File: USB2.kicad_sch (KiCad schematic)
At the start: 0 parts

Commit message: usb work cont
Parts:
- added P1: USB_C_Plug_USB2.0, symbol Connector:USB_C_Plug_USB2.0
- added U2: TUSB2046BIVFR, TUSB2046BIVFR:QFP80P900X900X145-32N, symbol TUSB2046BIVFR:TUSB2046BIVFR
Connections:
- new net: P1.A1 (GND), P1.A12 (GND), P1.B1 (GND), P1.B12 (GND)
- new net: P1.A4 (VBUS), P1.A9 (VBUS), P1.B4 (VBUS), P1.B9 (VBUS)
- new net USB2_HOST2_DM: U2.2 (DM0)
- new net USB2_HOST2_DP: U2.1 (DP0)

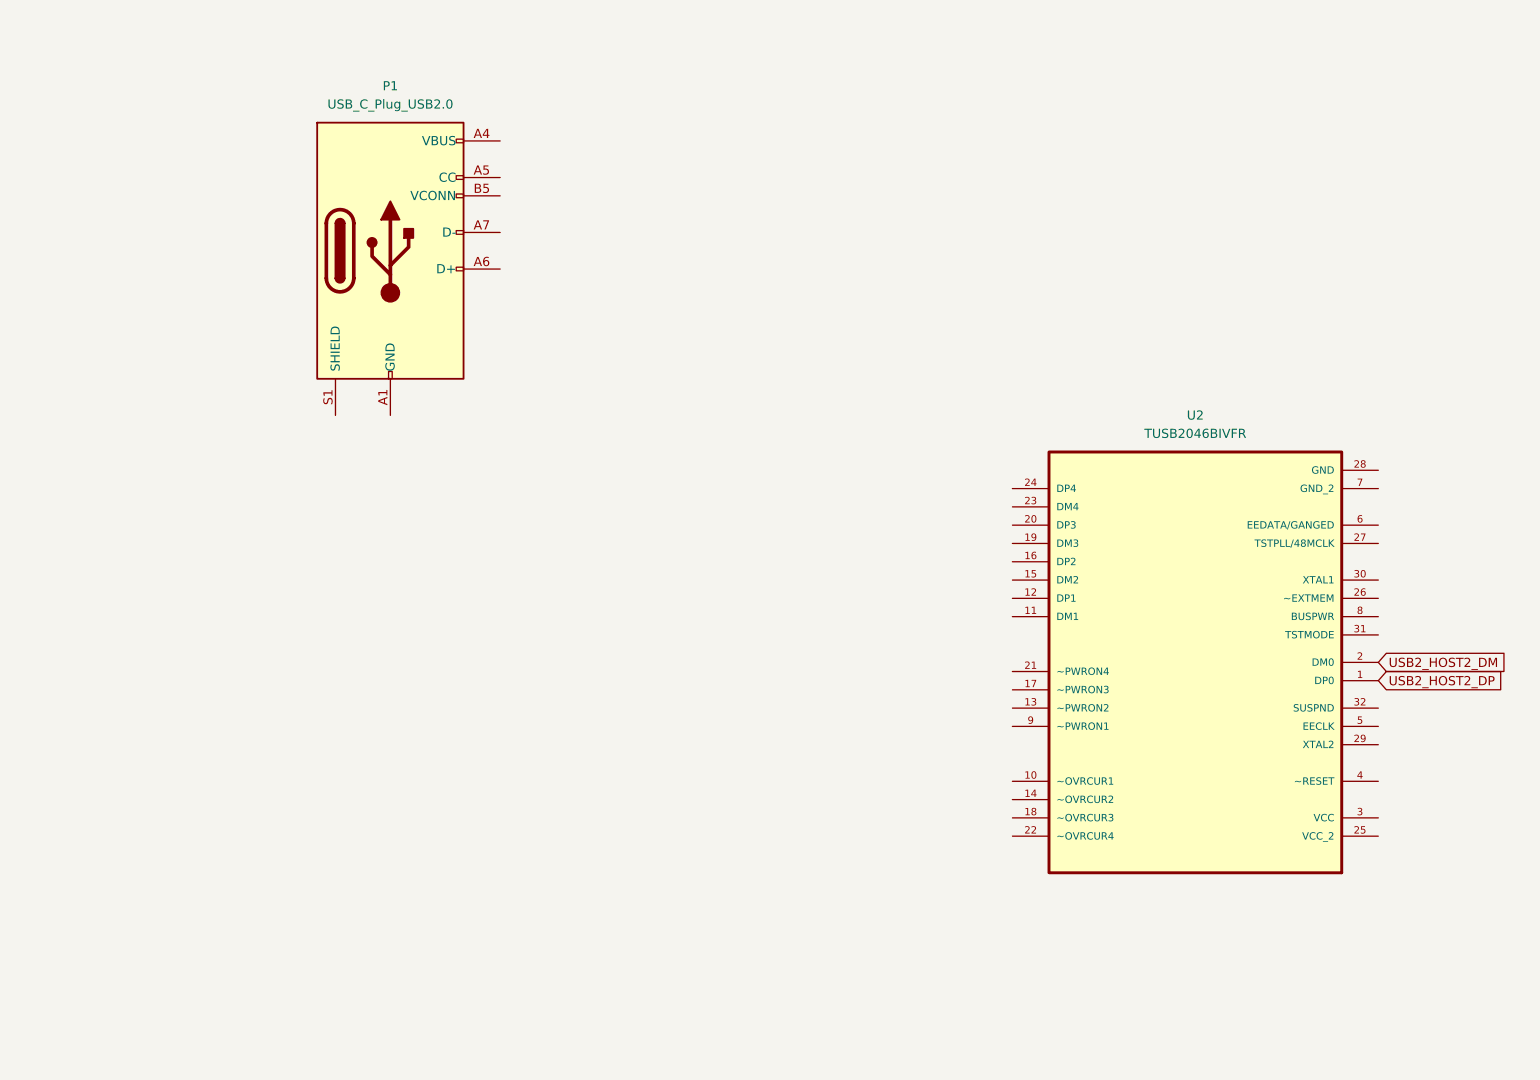
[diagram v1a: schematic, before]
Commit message: usb work cont
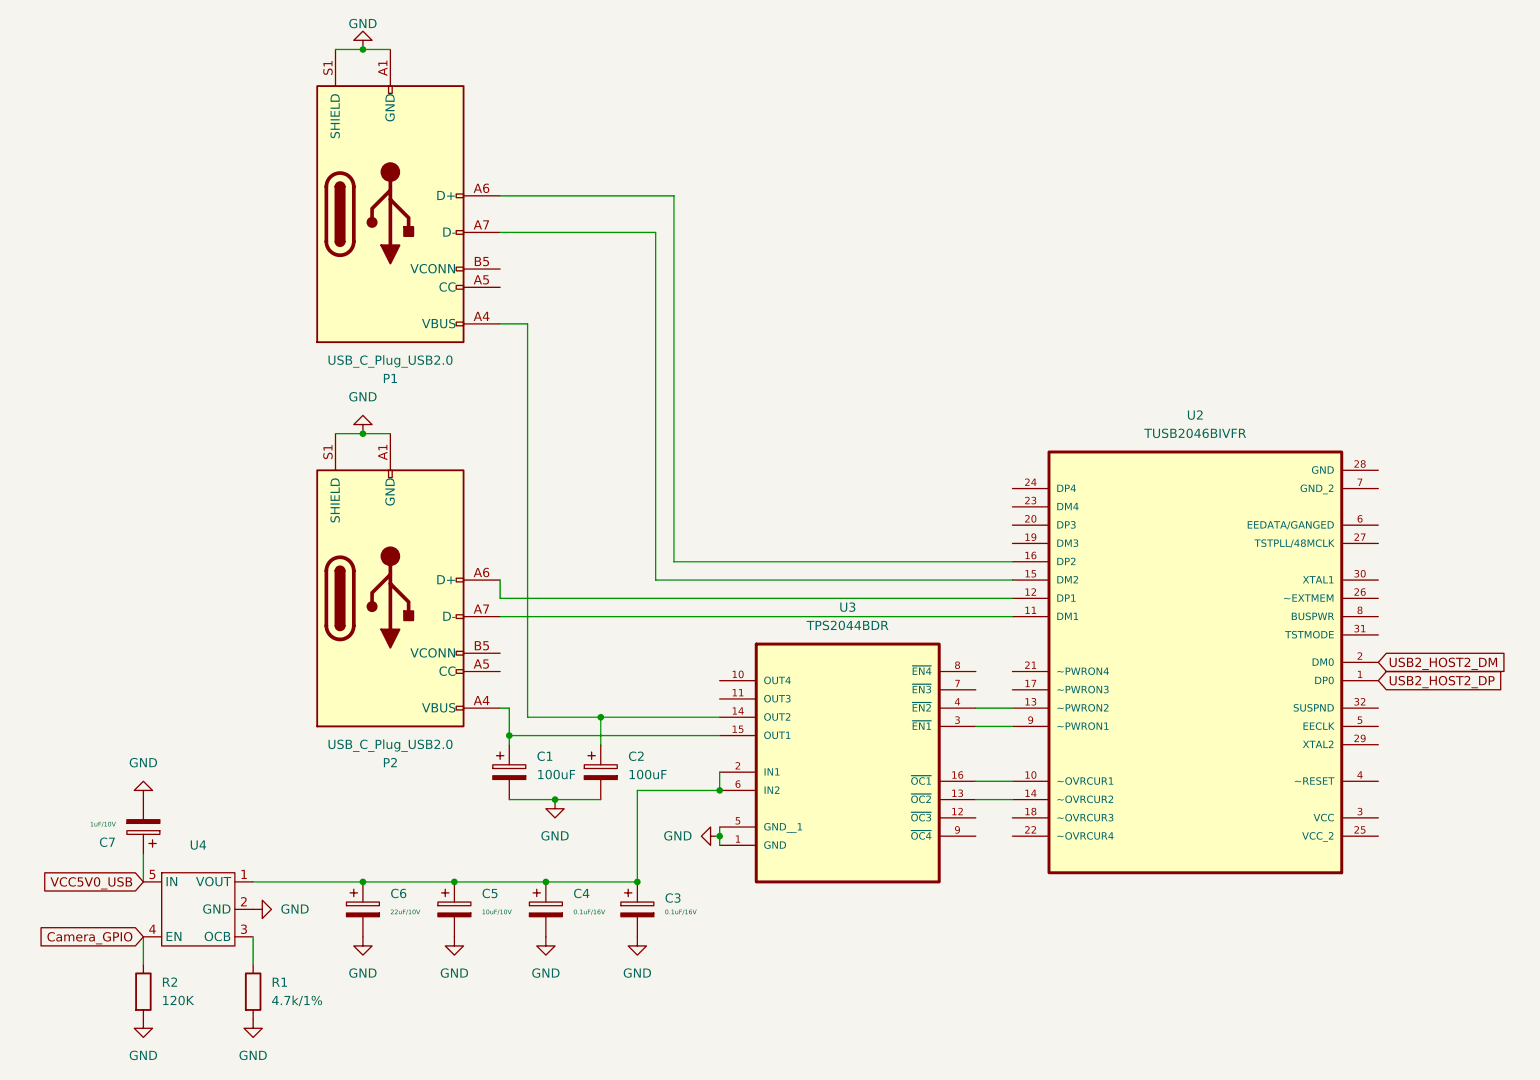
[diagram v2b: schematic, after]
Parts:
- added C1, C2: 100uF, symbol Device:C_Polarized
- added C3, C4: 0.1uF/16V, symbol Device:C_Polarized
- added C5: 10uF/10V, symbol Device:C_Polarized
- added C6: 22uF/10V, symbol Device:C_Polarized
- added C7: 1uF/10V, symbol Device:C_Polarized
- added P2: USB_C_Plug_USB2.0, symbol Connector:USB_C_Plug_USB2.0
- added R1: 4.7k/1%, symbol Device:R
- added R2: 120K, symbol Device:R
- added U3: TPS2044BDR, TPS2044BDR:SOIC127P600X175-16N, symbol TPS2044BDR:TPS2044BDR
- added U4: ~, symbol raxda:SGM2576YN5G/TR
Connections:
- net GND: now reaches P1.A1 (GND), P1.A12 (GND), P1.B1 (GND), P1.B12 (GND)
- net GND: now also P1.S1 (SHIELD), C1.2, C2.2, C3.2, C4.2, C5.2, C6.2, C7.2, P2.A1 (GND), P2.A12 (GND), P2.B1 (GND), P2.B12 (GND), P2.S1 (SHIELD), R1.2, R2.2, U3.1 (GND), U3.5 (GND__1), U4.2 (GND)
- net at P1.A4 (VBUS), P1.A9 (VBUS), P1.B4 (VBUS)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: now also C2.1, U3.14 (OUT2)
- net at P1.A6 (D+): now also U2.16 (DP2)
- net at P1.A7 (D-): now also U2.15 (DM2)
- net at U2.10 (~OVRCUR1): now also U3.16 (~{OC1})
- net at U2.11 (DM1): now also P2.A7 (D-)
- net at U2.12 (DP1): now also P2.A6 (D+)
- net at U2.13 (~PWRON2): now also U3.4 (~{EN2})
- net at U2.14 (~OVRCUR2): now also U3.13 (~{OC2})
- net at U2.9 (~PWRON1): now also U3.3 (~{EN1})
- new net: C1.1, P2.A4 (VBUS), P2.A9 (VBUS), P2.B4 (VBUS), P2.B9 (VBUS), U3.15 (OUT1)
- new net: C3.1, C4.1, C5.1, C6.1, U3.2 (IN1), U3.6 (IN2), U4.1 (VOUT)
- new net: R1.1, U4.3 (OCB)
- new net Camera_GPIO: R2.1, U4.4 (EN)
- new net VCC5V0_USB: C7.1, U4.5 (IN)
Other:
- moved on the sheet: P1
